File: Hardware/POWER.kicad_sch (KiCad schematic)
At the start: 88 parts, among them J201 Battery, J202 POWER IN, J203 5V_SEL, J204 E5V, SW201 START, U201 AP2112K-3.3, U203 AP2151W, U204 AP2112K-3.3, U205 AP2112K-1.8, U206 AP2112K-3.3, U207 AP2112K-3.3, U208 AP22814BW5

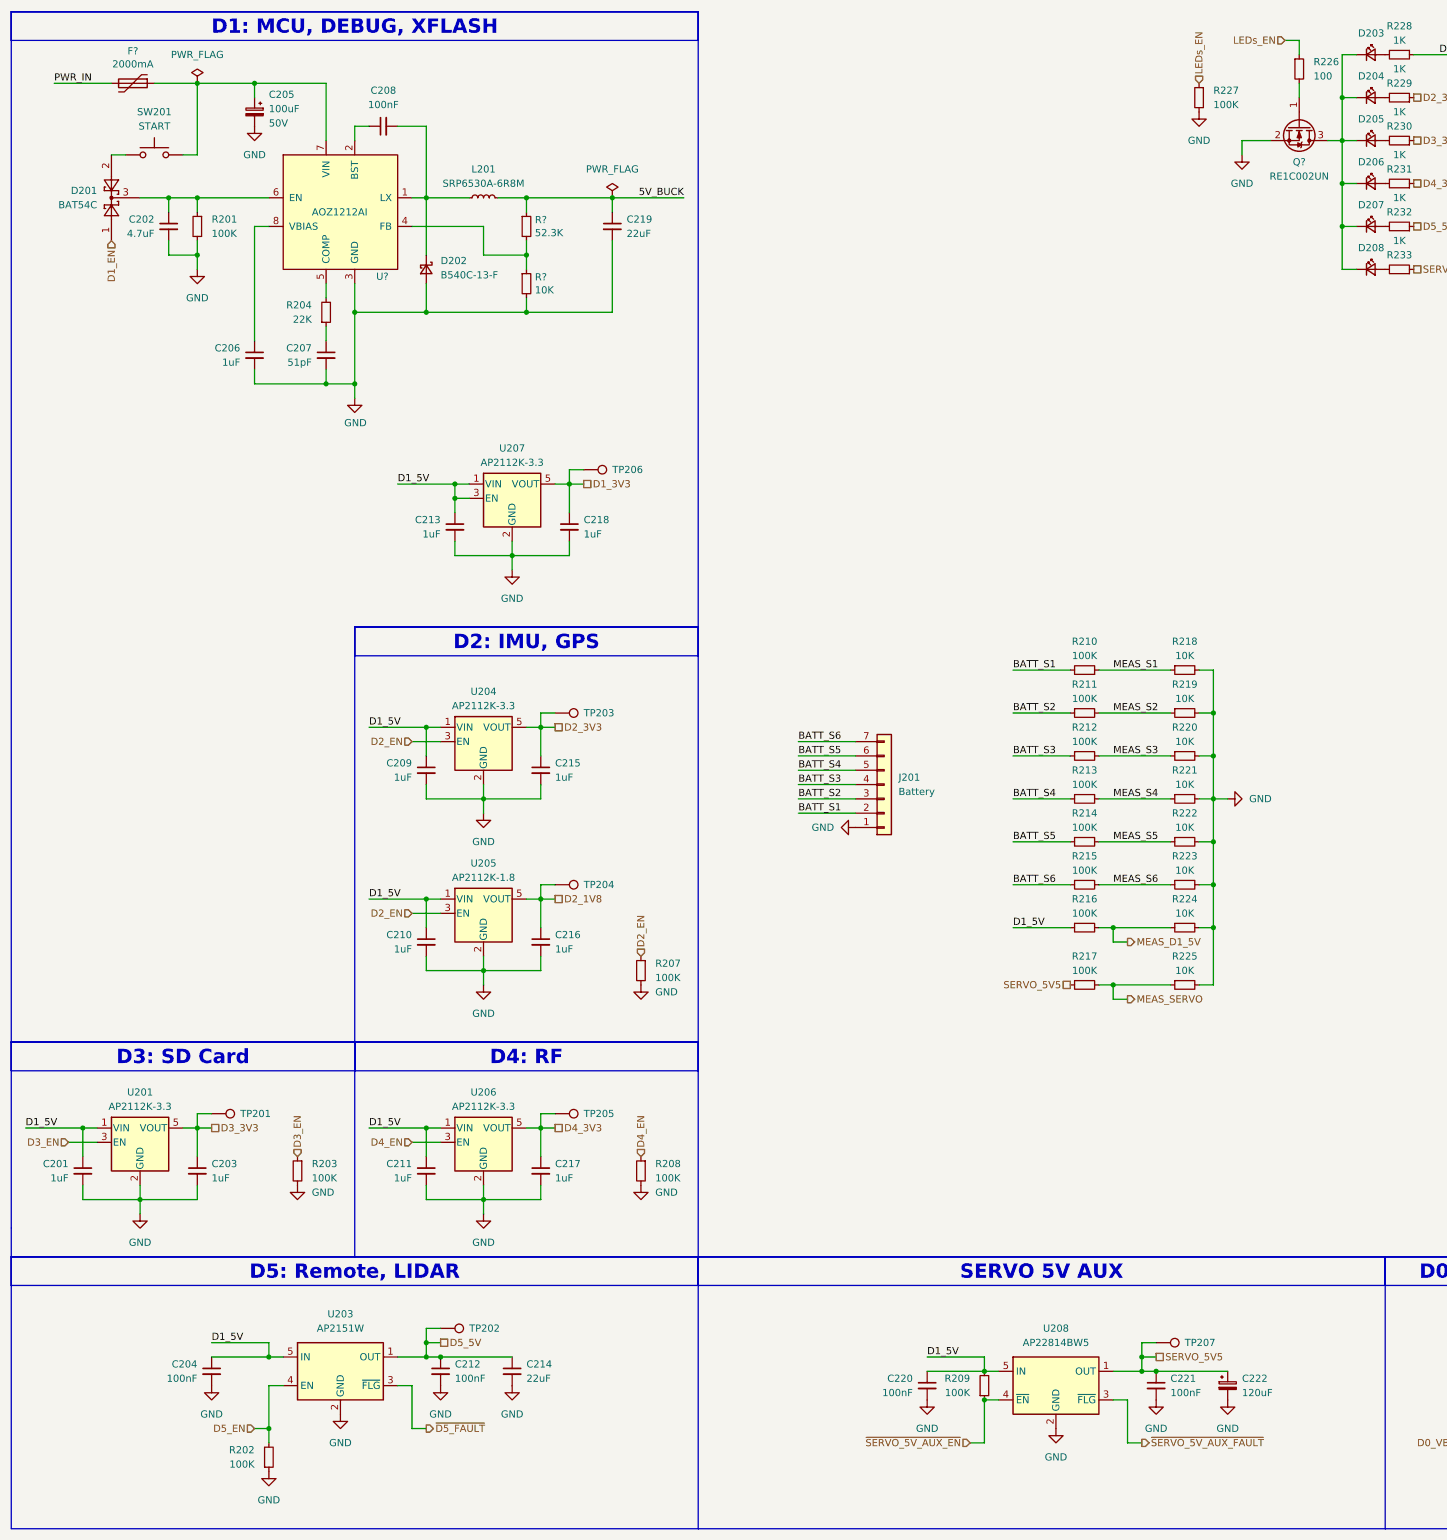
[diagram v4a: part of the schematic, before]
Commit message: Checkpoint
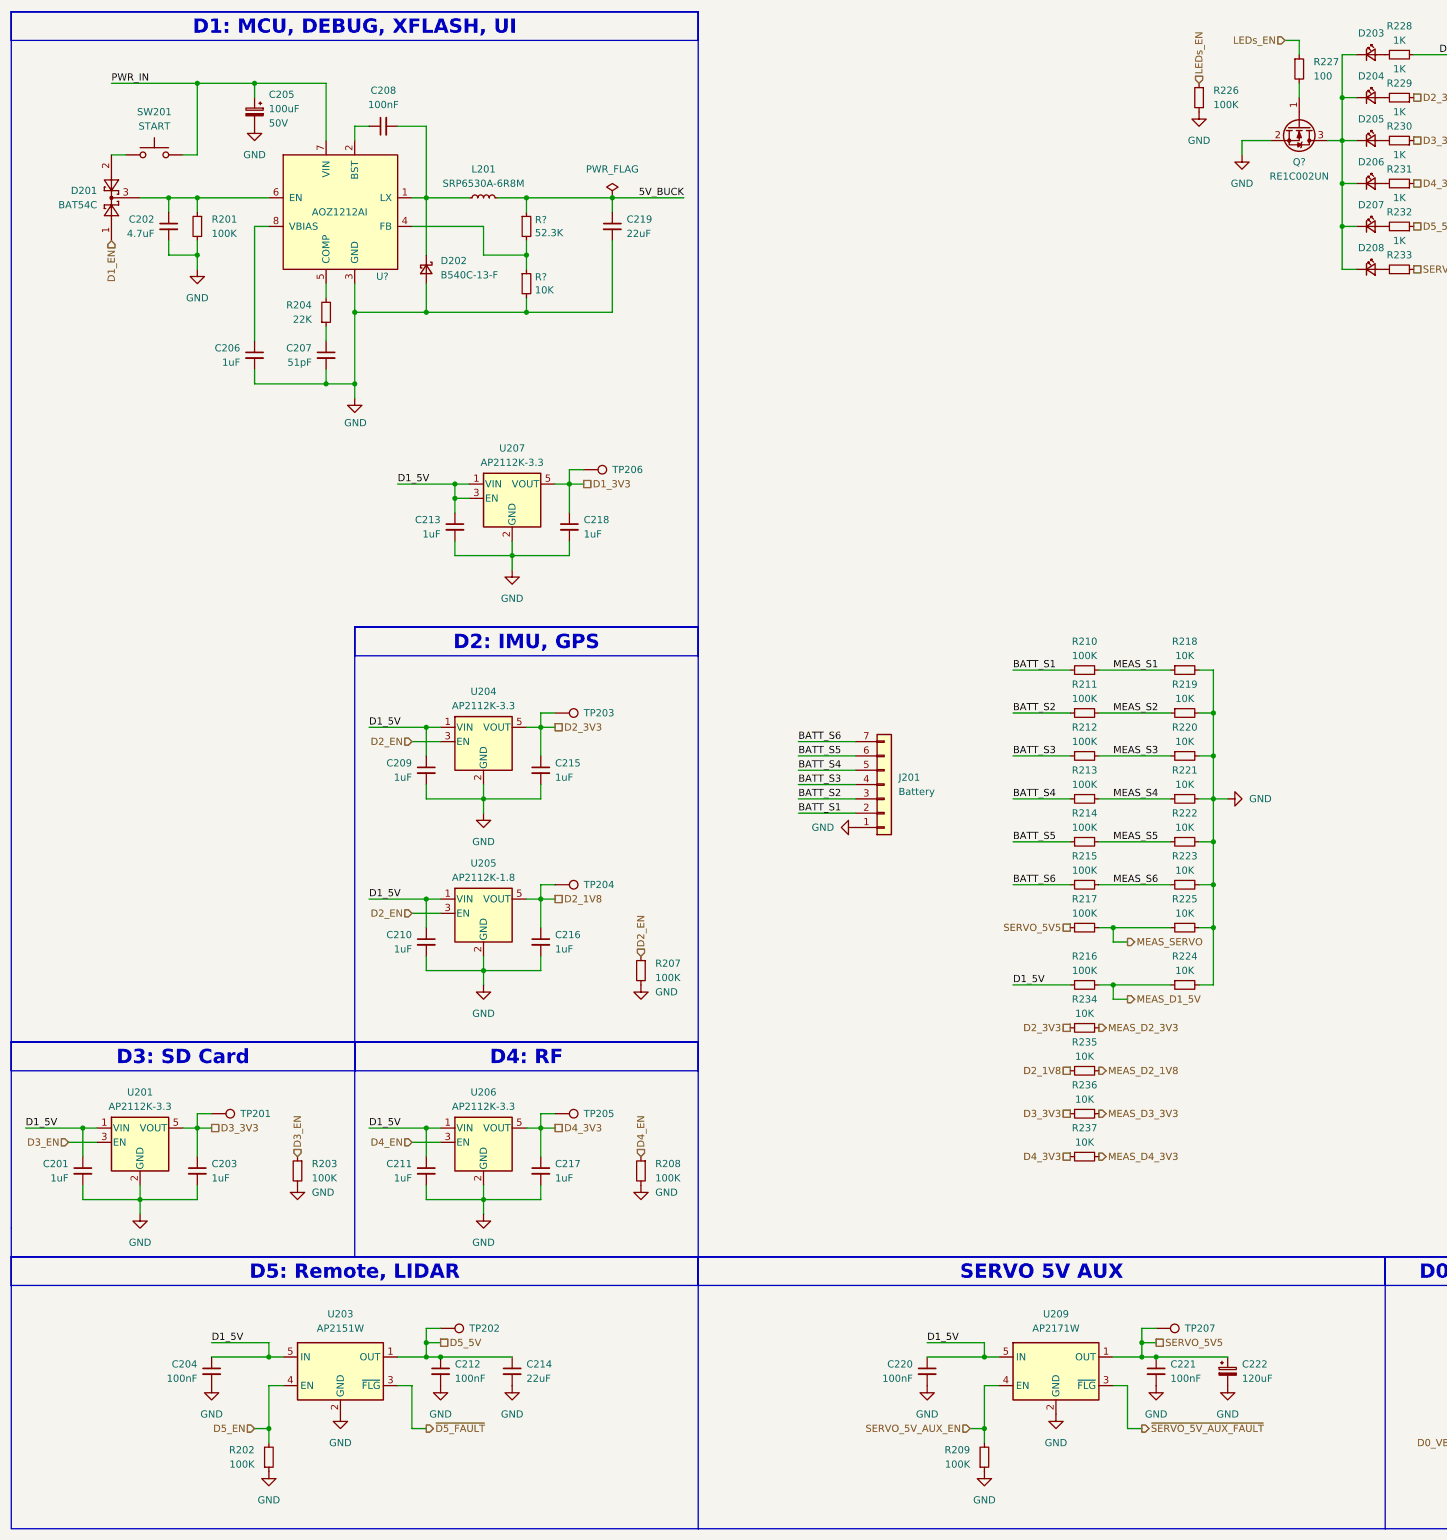
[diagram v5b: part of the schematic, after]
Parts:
- removed F?: 2000mA, Fuse:Fuse_1812_4532Metric, symbol Device:Polyfuse
- removed U208: AP22814BW5, Package_TO_SOT_SMD:SOT-23-5, symbol Power_Management:AP22814BW5
- added R234, R235, R236, R237: 10K, Resistor_SMD:R_0603_1608Metric, symbol Device:R_Small
- added U209: AP2171W, Package_TO_SOT_SMD:SOT-23-5, symbol Power_Management:AP2171W
- renumbered R227 to R226, R226 to R227
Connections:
- net ~{SERVO_5V_AUX_EN} is gone; now on net GND: R209.1
- net D1_5V: now also U209.5 (IN); no longer R209.2
- net D2_1V8: now also R235.1
- net D2_3V3: now also R234.1
- net D3_3V3: now also R236.1
- net D4_3V3: now also R237.1
- net GND: now also U209.2 (GND)
- net PWR_IN: now also C205.1, SW201.2, U?.7 (VIN)
- net SERVO_5V5: now also U209.1 (OUT)
- net ~{SERVO_5V_AUX_FAULT}: now also U209.3 (~{FLG})
- new net MEAS_D2_1V8: R235.2
- new net MEAS_D2_3V3: R234.2
- new net MEAS_D3_3V3: R236.2
- new net MEAS_D4_3V3: R237.2
- new net SERVO_5V_AUX_EN: R209.2, U209.4 (EN)
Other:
- moved on the sheet: C220, C221, C222, R209, R216, R217, R224, R225, TP207
